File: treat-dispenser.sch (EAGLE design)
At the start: 40 parts, among them U1 MCP73831, U2 TPS6103x, U3 ATMEGA32U4, Y1 16MHz

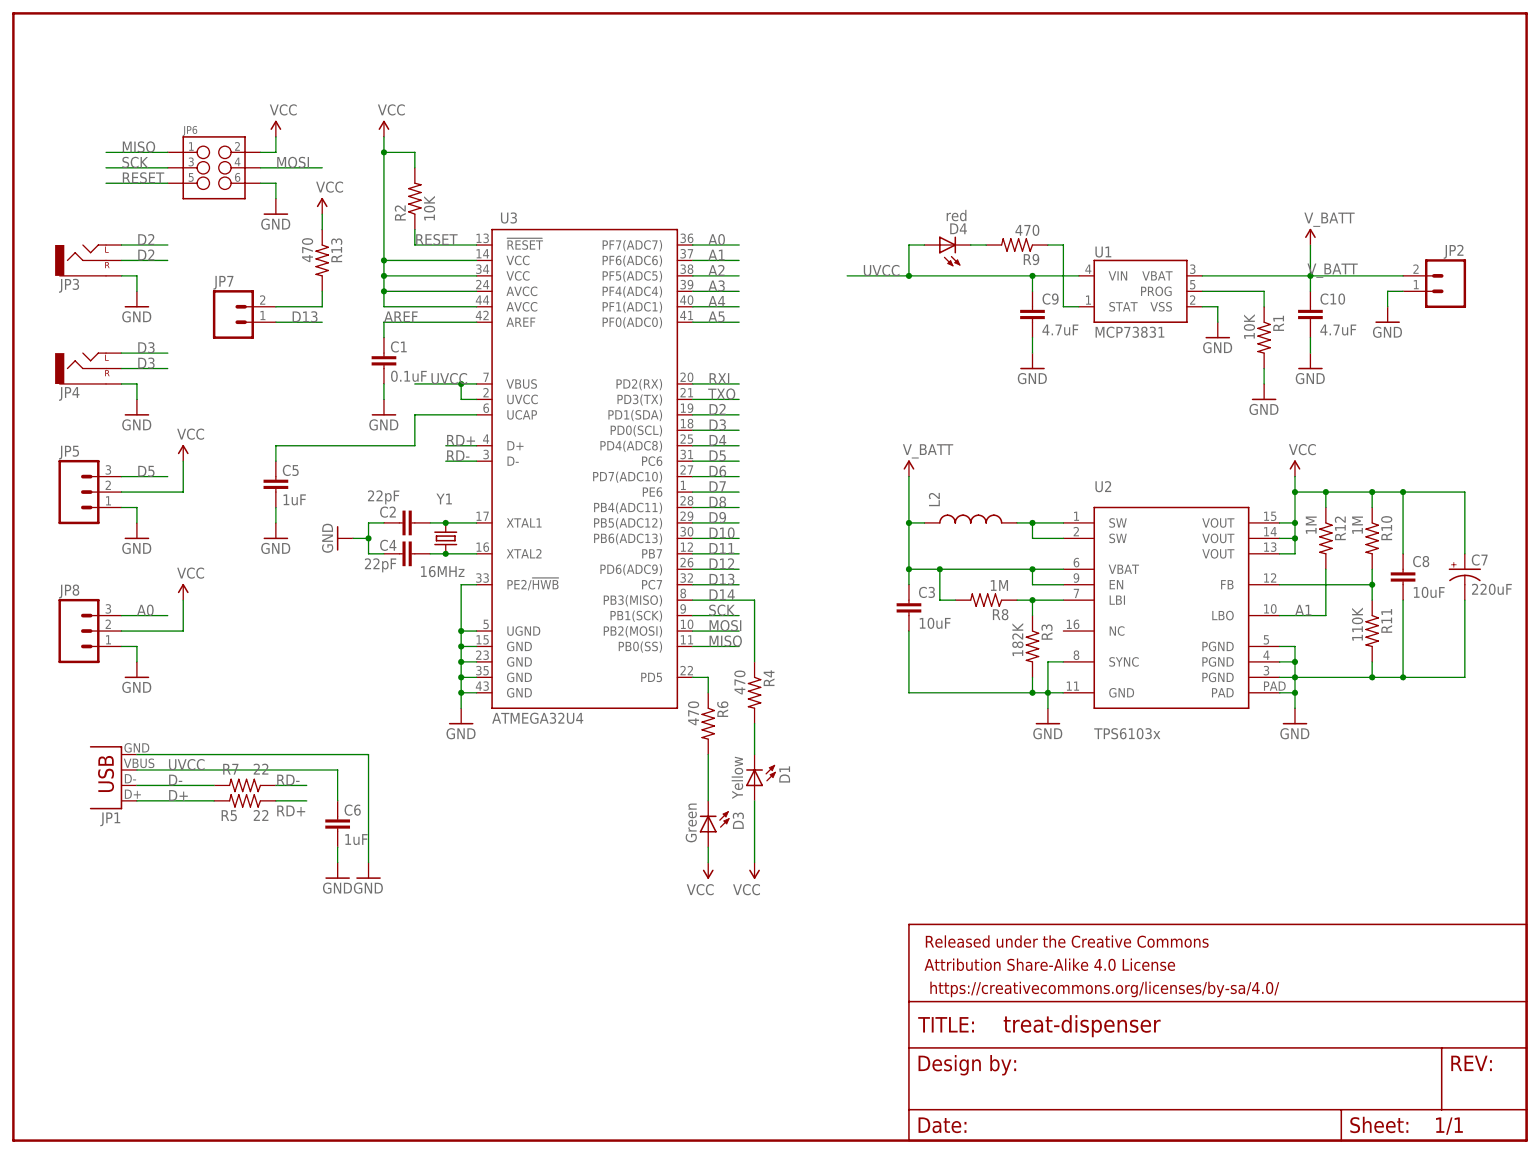
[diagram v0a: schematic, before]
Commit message: rev A initial commit
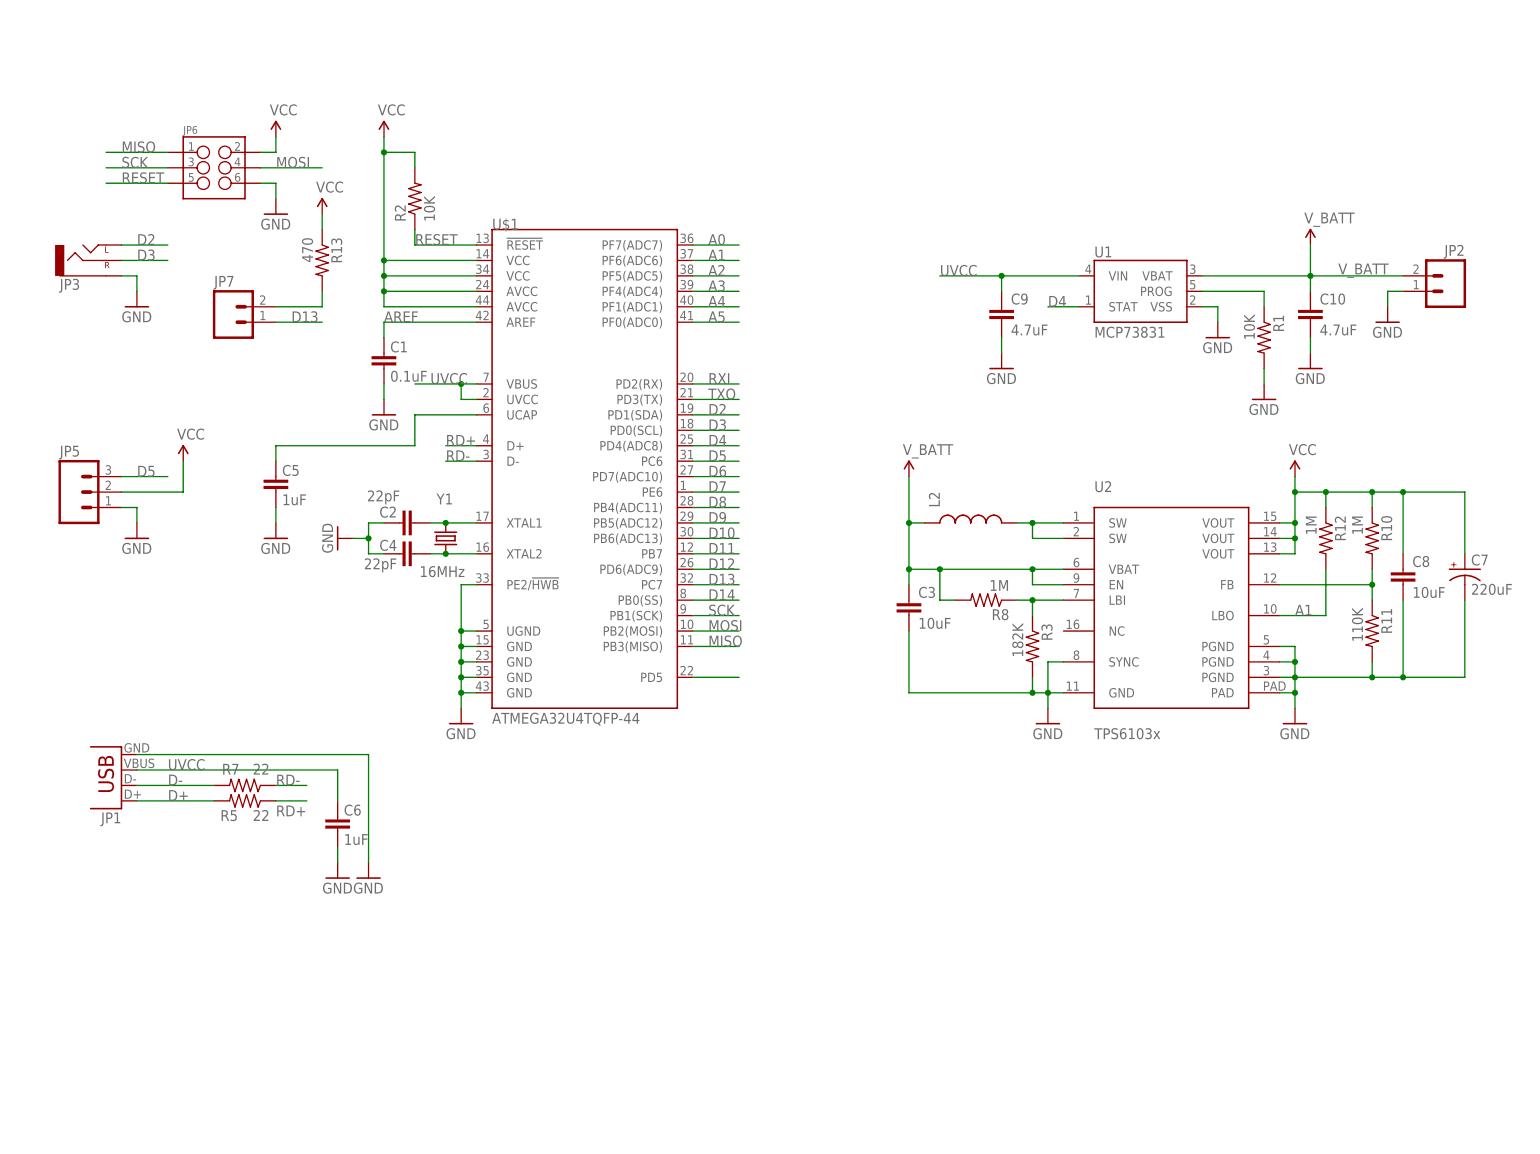
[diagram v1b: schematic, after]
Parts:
- removed D1: Yellow, SparkFun:LED0603
- removed D3: Green, SparkFun:LED0603
- removed D4: red, SparkFun:LED0603
- removed FRAME1: FRAME-LETTER, SparkFun-Aesthetics:FRAME-LETTER
- removed JP4: (no value), SparkFun-Connectors:AUDIO-JACKPTH
- removed JP8: (no value), SparkFun-Connectors:M03PTH
- removed R4, R6, R9: 470, SparkFun:RESISTOR0603-RES
- removed U3: ATMEGA32U4, Testing:ATMEGA32U4OUTFAKES
- added U$1: ATMEGA32U4TQFP-44, SparkFun-DigitalIC:ATMEGA32U4TQFP-44
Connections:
- removed net N$5: D1.C, R4.2
- removed net N$7: D3.C, R6.2
- removed net STAT: R9.1, U1.STAT
- removed net TXLED: R6.1, U3.PD5
- net A0: now also U$1.PF7(ADC7); no longer JP8.3, U3.PF7(ADC7)
- net A1: now also U$1.PF6(ADC6); no longer U3.PF6(ADC6)
- net A2: now also U$1.PF5(ADC5); no longer U3.PF5(ADC5)
- net A3: now also U$1.PF4(ADC4); no longer U3.PF4(ADC4)
- net A4: now also U$1.PF1(ADC1); no longer U3.PF1(ADC1)
- net A5: now also U$1.PF0(ADC0); no longer U3.PF0(ADC0)
- net AREF: now also U$1.AREF; no longer U3.AREF
- net D10: now also U$1.PB6(ADC13); no longer U3.PB6(ADC13)
- net D11: now also U$1.PB7; no longer U3.PB7
- net D12: now also U$1.PD6(ADC9); no longer U3.PD6(ADC9)
- net D13: now also U$1.PC7; no longer U3.PC7
- net D14: now also U$1.PB0(SS); no longer R4.1, U3.PB3(MISO)
- net D2: now also U$1.PD1(SDA); no longer JP3.RIGHT, U3.PD1(SDA)
- net D3: now also JP3.RIGHT, U$1.PD0(SCL); no longer JP4.LEFT, JP4.RIGHT, U3.PD0(SCL)
- net D4: now also U$1.PD4(ADC8), U1.STAT; no longer U3.PD4(ADC8)
- net D5: now also U$1.PC6; no longer U3.PC6
- net D6: now also U$1.PD7(ADC10); no longer U3.PD7(ADC10)
- net D7: now also U$1.PE6; no longer U3.PE6
- net D8: now also U$1.PB4(ADC11); no longer U3.PB4(ADC11)
- net D9: now also U$1.PB5(ADC12); no longer U3.PB5(ADC12)
- net GND: now also U$1.GND@15, U$1.GND@23, U$1.GND@35, U$1.GND@43, U$1.PE2/!HWB, U$1.UGND; no longer JP4.SLEEVE, JP8.1, U3.GND@15, U3.GND@23, U3.GND@35, U3.GND@43, U3.PE2/!HWB, U3.UGND
- net MISO: now also U$1.PB3(MISO); no longer U3.PB0(SS)
- net MOSI: now also U$1.PB2(MOSI); no longer U3.PB2(MOSI)
- net N$1: now also U$1.XTAL2; no longer U3.XTAL2
- net N$2: now also U$1.XTAL1; no longer U3.XTAL1
- net N$3: now also U$1.PD5; no longer D4.C, R9.2
- net N$4: now also U$1.UCAP; no longer U3.UCAP
- net RD+: now also U$1.D+; no longer U3.D+
- net RD-: now also U$1.D-; no longer U3.D-
- net RESET: now also U$1.!RESET; no longer U3.!RESET
- net RXI: now also U$1.PD2(RX); no longer U3.PD2(RX)
- net SCK: now also U$1.PB1(SCK); no longer U3.PB1(SCK)
- net TXO: now also U$1.PD3(TX); no longer U3.PD3(TX)
- net UVCC: now also U$1.UVCC, U$1.VBUS; no longer D4.A, U3.UVCC, U3.VBUS
- net VCC: now also U$1.AVCC@24, U$1.AVCC@44, U$1.VCC@14, U$1.VCC@34; no longer D1.A, D3.A, JP8.2, U3.AVCC@24, U3.AVCC@44, U3.VCC@14, U3.VCC@34
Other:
- moved on the sheet: C9
